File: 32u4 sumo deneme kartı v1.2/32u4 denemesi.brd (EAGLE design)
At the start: 100 x 100 mm, 136 parts, among them IC1 IC_555-SOIC8, IC2 LM2577S, IC3 LMV358MX, J1 AVR_SPI_PRG_6NS, Q2 SI3456BDVSOT-5-6, U1 TB6612FNG

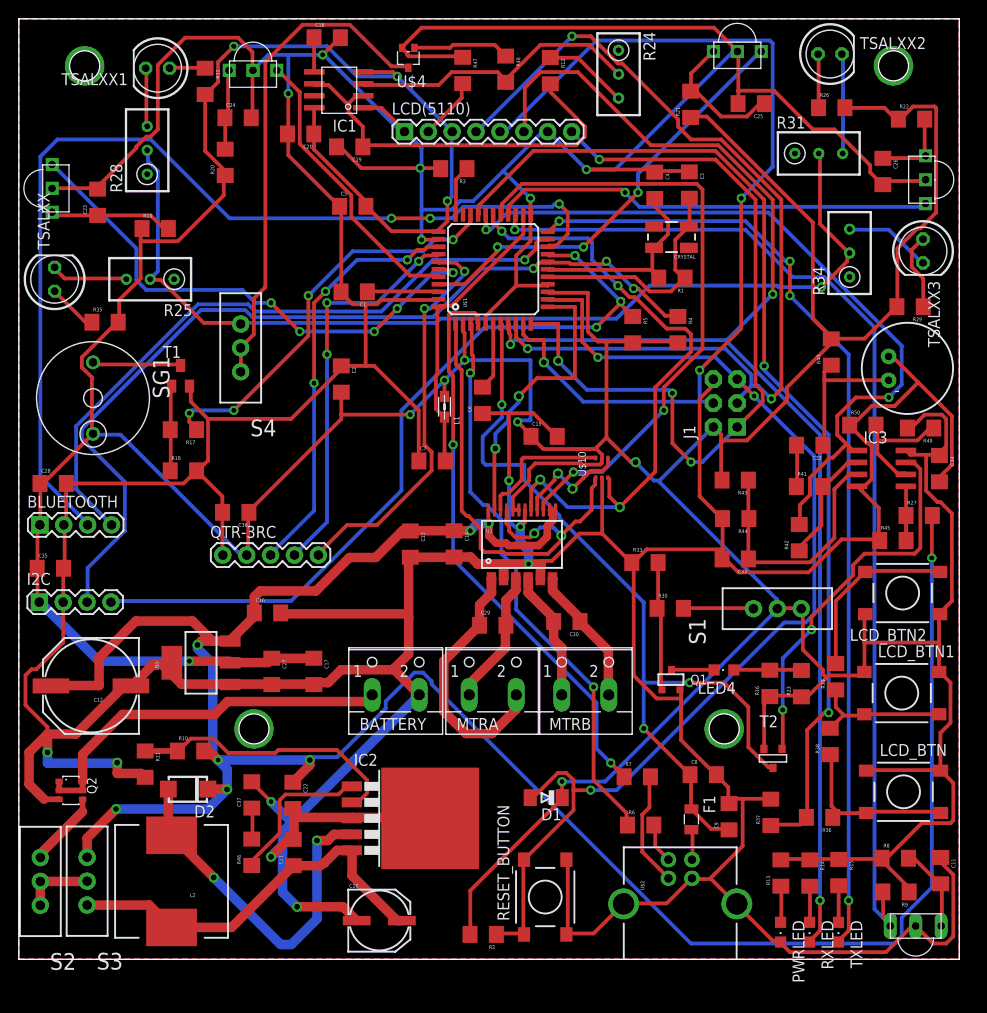
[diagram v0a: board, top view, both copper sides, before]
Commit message: ver1.4
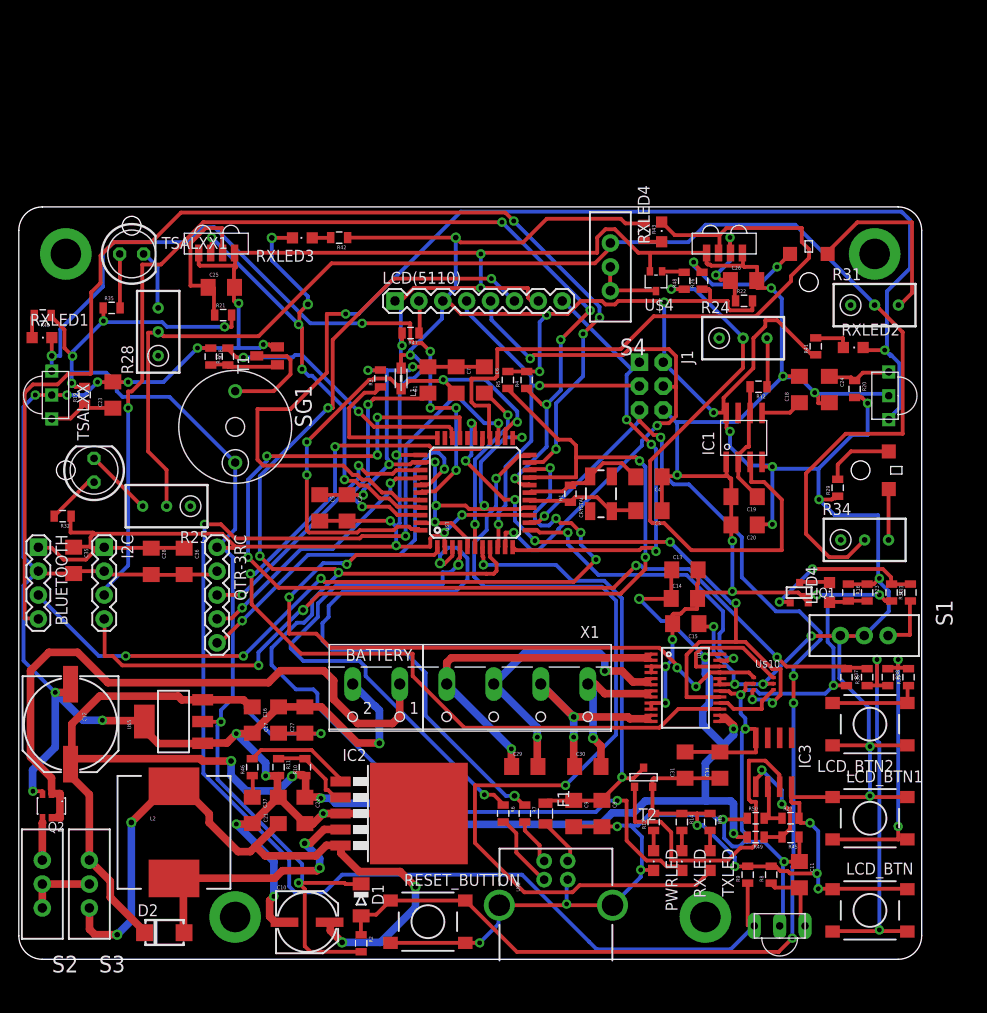
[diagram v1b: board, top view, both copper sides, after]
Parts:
- removed C32, C33: 4.7uF, SparkFun-Passives:1206
- removed MTRA, MTRB: (no value), con-wago-500:W237-102
- removed R44: 10k, SparkFun-Resistors:1206
- removed TSALXX2, TSALXX3: (no value), led:LED5MM
- removed U$13: MIC9.7MM, SparkFun-Sensors:MIC-9.7MM
- added C31: 100nF, SparkFun-Passives:1206
- added RXLED1, RXLED2, RXLED3, RXLED4: (no value), led:CHIPLED_0805
- added U$11, U$12: IRLED, HACIBİDEAS:IRLED
- added X1: (no value), con-wago-500:W237-4
- R1: device SparkFun-Resistors:1206 -> SparkFun-Resistors:0805
- R10: value 10.5k -> 10.5K; device SparkFun-Resistors:1206 -> SparkFun-Resistors:0805
- R11: value 2k -> 2K; device SparkFun-Resistors:1206 -> SparkFun-Resistors:0805
- R12: value 39.2 -> 39.2K; device SparkFun-Resistors:1206 -> SparkFun-Resistors:0805
- R13, R47: value 220 -> 220R; device SparkFun-Resistors:1206 -> SparkFun-Resistors:0805
- R14, R15, R16, R17, R23, R36: value 1k -> 1K; device SparkFun-Resistors:1206 -> SparkFun-Resistors:0805
- R18, R2, R3, R30, R37, R45: value 10k -> 10K; device SparkFun-Resistors:1206 -> SparkFun-Resistors:0805
- R19, R20, R21, R22, R48: value 100 -> 100R; device SparkFun-Resistors:1206 -> SparkFun-Resistors:0805
- R26, R29, R32, R35, R8: value 47 -> 47R; device SparkFun-Resistors:1206 -> SparkFun-Resistors:0805
- R27, R4, R49, R5: value 4.7k -> 4.7K; device SparkFun-Resistors:1206 -> SparkFun-Resistors:0805
- R33: value 47k -> 47K; device SparkFun-Resistors:1206 -> SparkFun-Resistors:0805
- R38: value 7.5k -> 7.5K; device SparkFun-Resistors:1206 -> SparkFun-Resistors:0805
- R39: value 68k -> 68K; device SparkFun-Resistors:1206 -> SparkFun-Resistors:0805
- R40: value 2.2k -> 1K; device SparkFun-Resistors:1206 -> SparkFun-Resistors:0805
- R41, R43: value 10k -> 1K; device SparkFun-Resistors:1206 -> SparkFun-Resistors:0805
- R42: value 820 -> 1K; device SparkFun-Resistors:1206 -> SparkFun-Resistors:0805
- R46, R50: value 2.2k -> 2.2K; device SparkFun-Resistors:1206 -> SparkFun-Resistors:0805
- R6, R7: value 22 -> 22R; device SparkFun-Resistors:1206 -> SparkFun-Resistors:0805
- R9: value 20k -> 20K; device SparkFun-Resistors:1206 -> SparkFun-Resistors:0805
- U$6, U$7: value TSSPXX38 -> TSSP7P38; device HACIBİDEAS:TSSPXX38 -> HACIBİDEAS:TSSP7P38
- moved R40 83.9 mm to (2.54, 68.5), turned to 180 degrees
- moved U$6 76.6 mm to (21.0, 75.0), turned to 180 degrees
- moved U$8 76.3 mm to (93.5, 57.4), turned to 90 degrees
- moved R20 71.1 mm to (88.9, 60.6), turned to 270 degrees
- moved C24 69.2 mm to (86.2, 60.6), turned to 270 degrees
- moved C20 62.9 mm to (77.1, 46.2)
- moved C18 62.6 mm to (83.0, 60.6), turned to 90 degrees
- moved C25 59.6 mm to (21.5, 71.4), turned to 0 degrees
- moved R42 58.4 mm to (34.1, 76.7), turned to 180 degrees
- moved IC1 56.8 mm to (77.1, 55.5), turned to 0 degrees
- moved C19 56.1 mm to (77.1, 49.2)
- moved R21 54.5 mm to (21.7, 68.5), turned to 0 degrees
- moved R32 48.6 mm to (4.66, 47.1), turned to 180 degrees
- moved R49 46.9 mm to (78.3, 13.0)
- moved R50 43.3 mm to (78.3, 15.0)
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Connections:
- removed net N$19: C32.1, R40.1, U$13.2
- removed net N$20: C32.2, R41.1
- new net N$30: R41.2, RXLED2.A
- new net N$56: R43.2, RXLED4.A
- net +5V: now also C31.1, QTR-3RC.1, R19.2, R20.2, R21.2, R22.2, R26.1, R27.2, R29.1, R32.1, R35.1, R40.1, R41.1, R42.1, R43.1, R8.2, R9.2; no longer QTR-3RC.2, R19.1, R20.1, R21.1, R22.1, R26.2, R29.2, R32.2, R35.2, R40.2, R43.2, R49.2, R8.1, R9.1
- net 38KHZOUT: now also R48.1; no longer R48.2
- net A01: now also X1.4; no longer MTRA.2
- net A02: now also X1.3; no longer MTRA.1
- net A3: now also RXLED1.C
- net A4: now also RXLED2.C
- net A5: now also RXLED3.C, U$6.3; no longer U$7.OUT
- net B01: now also X1.2; no longer MTRB.2
- net B02: now also X1.1; no longer MTRB.1
- net D+: now also R6.1; no longer R7.1
- net D-: now also R7.1; no longer R6.1
- net D12: now also RXLED4.C, U$7.3; no longer U$6.OUT
- net D4: now also R9.1; no longer R9.2
- net D5: now also R17.2; no longer R17.1
- net D9: no longer IC3.1, R42.2
- net GND: now also C31.2, QTR-3RC.2, R18.1, R33.2, R47.2, U$6.1, U$6.4, U$7.1, U$7.4; no longer C33.2, QTR-3RC.1, R18.2, R33.1, R44.2, R47.1, U$13.1, U$6.GND, U$7.GND
- net N$10: now also R6.2; no longer R7.2
- net N$11: now also R49.1; no longer R27.1
- net N$12: now also R8.1; no longer R8.2
- net N$15: now also R10.2; no longer R10.1
- net N$16: now also R48.2; no longer R48.1
- net N$17: now also R38.2; no longer R38.1
- net N$18: now also R38.1, R39.2; no longer R38.2, R39.1
- net N$21: now also R40.2, RXLED1.A; no longer IC3.2, R41.2, R42.1
- net N$25: now also R17.1, R18.2; no longer R17.2, R18.1
- net N$26: now also R27.1; no longer R49.1
- net N$34: now also R32.2; no longer R35.1
- net N$38: now also R35.2; no longer R32.1
- net N$39: now also R30.1; no longer R30.2
- net N$40: now also R30.2, R33.1; no longer R30.1, R33.2
- net N$41: now also U$11.P$1; no longer TSALXX2.K
- net N$42: now also R26.2, U$11.P$2; no longer R26.1, TSALXX2.A
- net N$45: now also U$12.P$1; no longer TSALXX3.K
- net N$46: now also R29.2, U$12.P$2; no longer R29.1, TSALXX3.A
- net N$50: now also R42.2, RXLED3.A; no longer C33.1, IC3.3, R43.1, R44.1
- net N$52: now also R46.2; no longer R46.1
- net N$53: now also R46.1; no longer R46.2
- net N$55: now also R47.1; no longer R47.2
- net N$8: now also R39.1; no longer R39.2
- net N$9: now also R7.2; no longer R6.2
- net VS1: now also R19.1; no longer R19.2
- net VS2: now also R20.1; no longer R20.2
- net VS3: now also R21.1, U$6.2; no longer R21.2, U$7.VS
- net VS4: now also R22.1, U$7.2; no longer R22.2, U$6.VS
- net V_BATT: now also R10.1, R49.2; no longer R10.2, R27.2
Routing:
- net GND: track 827.6 -> 630.6 mm, vias 14 -> 48
- net A4: track 30.8 -> 132.8 mm, vias 0 -> 2
- net V_BATT: track 252.8 -> 169.8 mm, vias 8 -> 7
- net D9: track 80.4 -> 0.00 mm, vias 2 -> 0
- net SCK: track 100.4 -> 42.0 mm, vias 3 -> 2
- net TX: track 71.5 -> 125.9 mm, vias 1 -> 4
- net N$31: track 52.8 -> 7.48 mm
- net +5V: track 618.1 -> 575.4 mm, vias 10 -> 35
- net MOSI: track 100.3 -> 58.6 mm
- net DRAIN: track 106.6 -> 146.9 mm, vias 1 -> 0
- net VUSB: track 89.1 -> 49.5 mm, vias 3 -> 2
- net D4: track 112.5 -> 148.7 mm, vias 1 -> 3
- net MISO: track 83.2 -> 49.1 mm, vias 4 -> 3
- net VIN: track 43.1 -> 74.5 mm, vias 0 -> 4
- net 38KHZOUT: track 31.5 -> 61.7 mm, vias 0 -> 1
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- removed copper zone on layer 1, net GND
- removed copper zone on layer 16, net GND
- removed copper zone on layer 1, net N$30
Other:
- board size 100 x 100 mm -> 96 x 80 mm
